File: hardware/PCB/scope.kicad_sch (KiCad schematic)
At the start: 21 parts, among them J10 Conn_Coaxial, U19 AD9283, Y2 50MHz

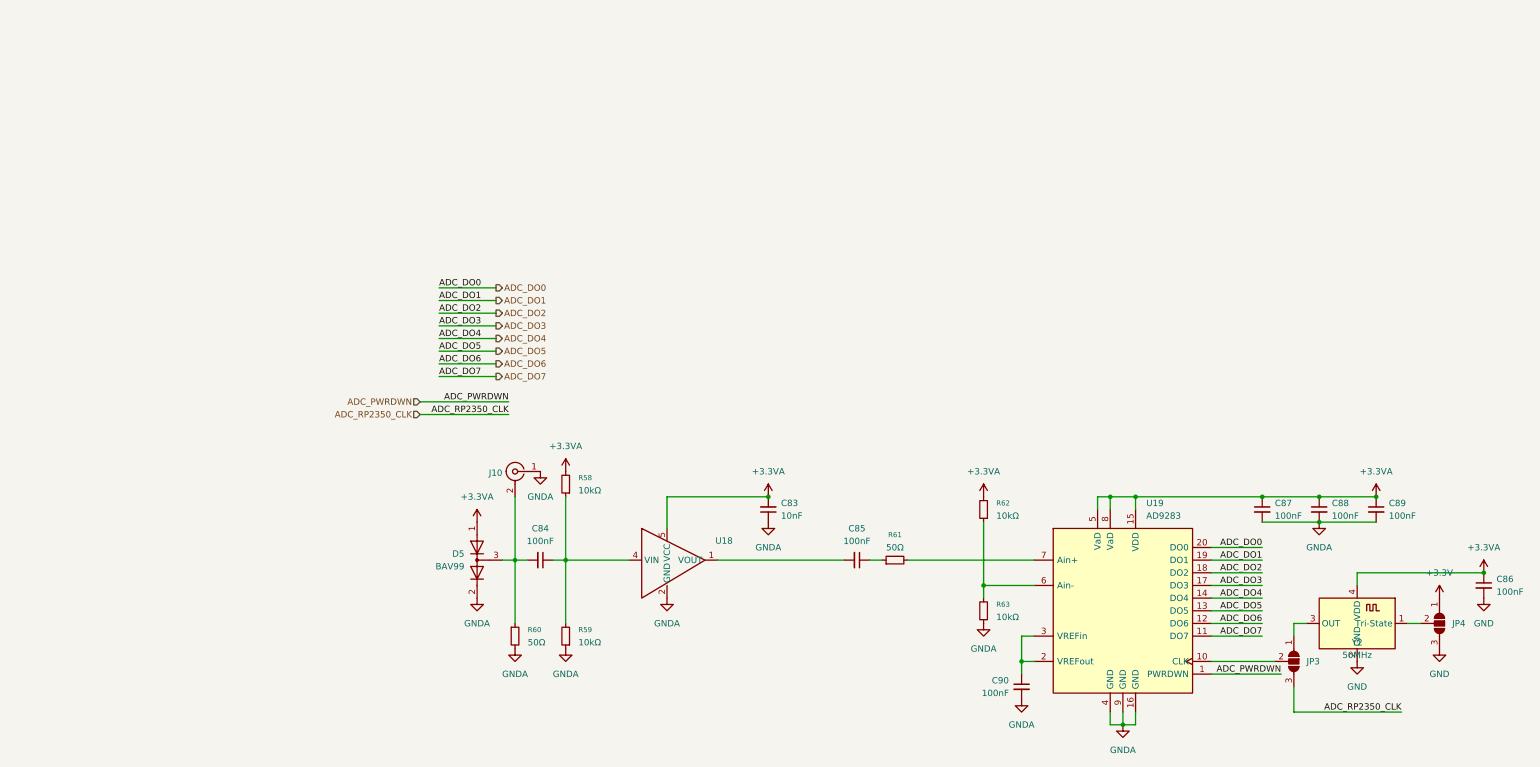
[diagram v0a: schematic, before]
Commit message: Completed schematic
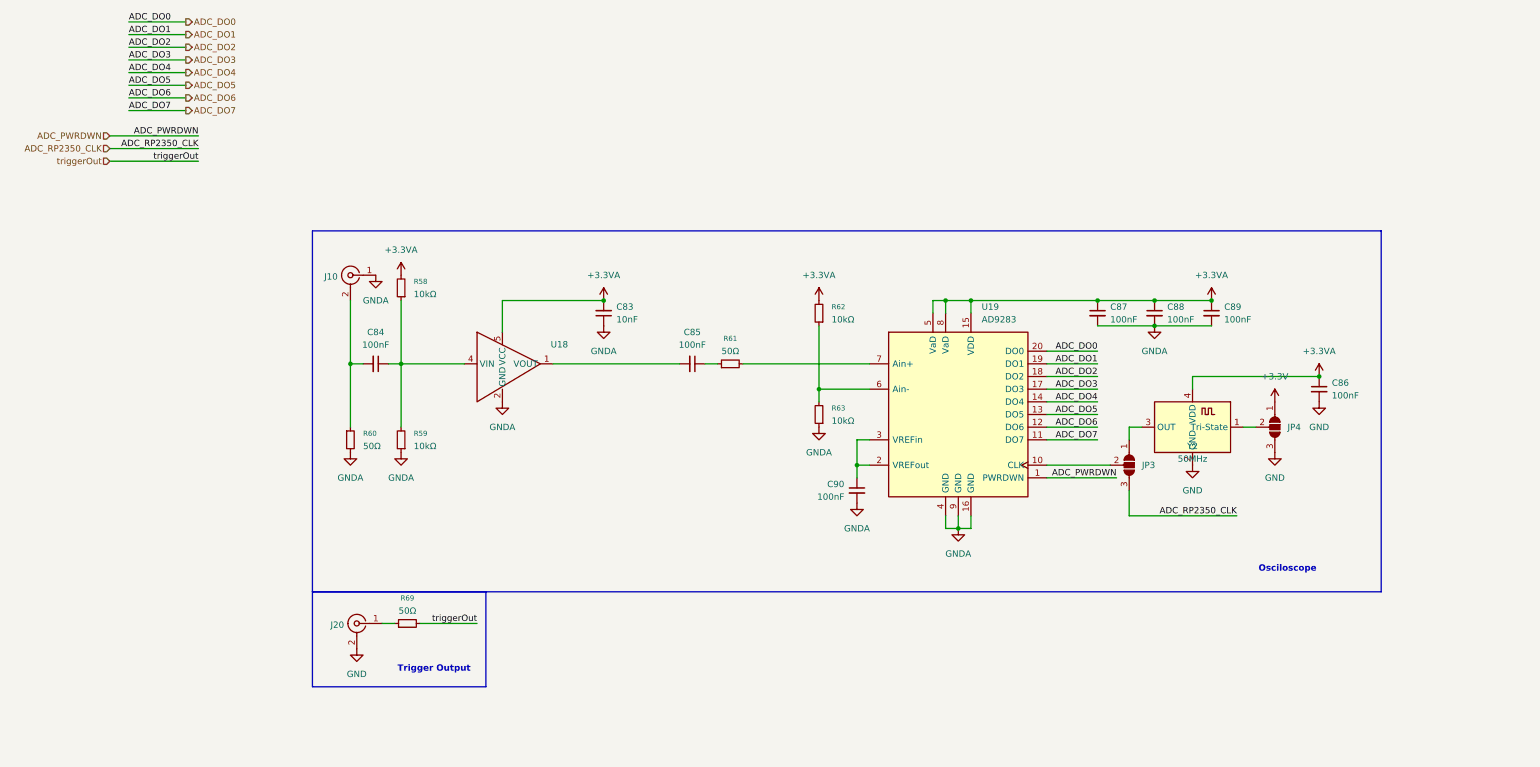
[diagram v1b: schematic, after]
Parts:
- removed D5: BAV99, Package_TO_SOT_SMD:SOT-23, symbol Diode:BAV99
- added J20: Conn_Coaxial, KiCad Libraries:TE_5227661-1, symbol Connector:Conn_Coaxial
- added R69: 50Ω, Resistor_SMD:R_0603_1608Metric_Pad0.98x0.95mm_HandSolder, symbol Device:R_Small
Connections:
- net GND: now also J20.2 (Ext)
- new net: J20.1 (In), R69.1
- new net triggerOut: R69.2
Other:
- note added: "Osciloscope"
- note added: "Trigger Output"
- moved on the sheet: C83, C84, C85, C86, C87, C88, C89, C90, J10, JP3, JP4, R58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
